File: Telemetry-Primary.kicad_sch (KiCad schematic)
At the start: 43 parts, among them J10 SDCard_LogicAnalyzer, J13 GPS_LogicAnalyzer, J5 SWD, J6 Breakouts, J7 CAN_LogicAnalyzer, J7 RTC_BATT, J8 CAN_LogicAnalyzer, SW1 Reset, U9 STM32F429ZITx, Y2 8M, Y3 32.768k

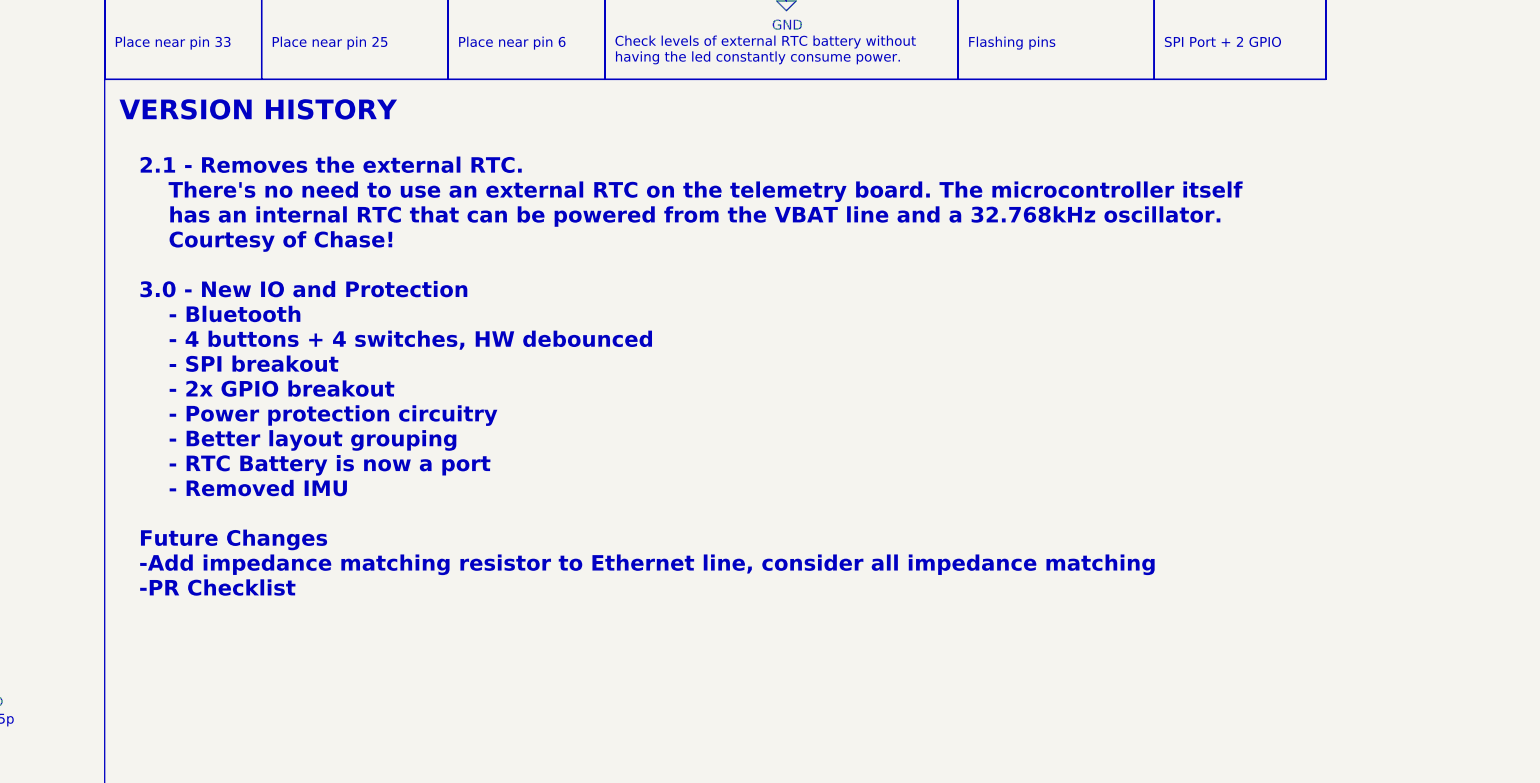
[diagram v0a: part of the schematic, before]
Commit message: silk screen cleanup + comments
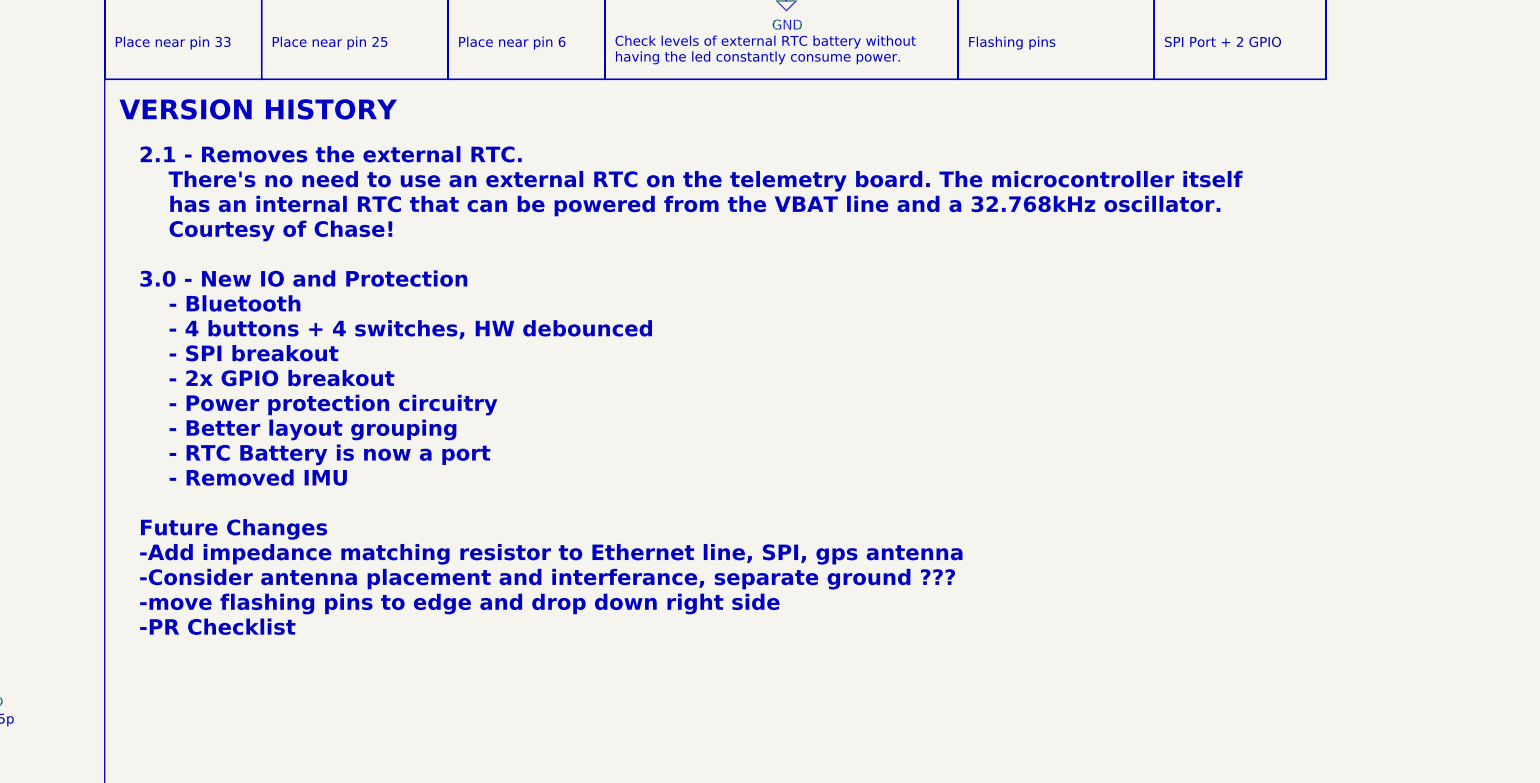
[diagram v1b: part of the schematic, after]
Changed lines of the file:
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@@
     (effects (font (size 1.27 1.27)) (justify left bottom))
   )
-  (text "2.1 - Removes the external RTC.\n	There's no need to use an external RTC on the telemetry board. The microcontroller itself\n	has an internal RTC that can be powered from the VBAT line and a 32.768kHz oscillator. \n	Courtesy of Chase!\n\n3.0 - New IO and Protection\n	- Bluetooth\n	- 4 buttons + 4 switches, HW debounced\n	- SPI breakout\n	- 2x GPIO breakout\n	- Power protection circuitry\n	- Better layout grouping\n	- RTC Battery is now a port\n	- Removed IMU\n\nFuture Changes\n-Add impedance matching resistor to Ethernet line, consider all impedance matching\n-PR Checklist"
-    (at 254 158.115 0)
+  (text "2.1 - Removes the external RTC.\n	There's no need to use an external RTC on the telemetry board. The microcontroller itself\n	has an internal RTC that can be powered from the VBAT line and a 32.768kHz oscillator. \n	Courtesy of Chase!\n\n3.0 - New IO and Protection\n	- Bluetooth\n	- 4 buttons + 4 switches, HW debounced\n	- SPI breakout\n	- 2x GPIO breakout\n	- Power protection circuitry\n	- Better layout grouping\n	- RTC Battery is now a port\n	- Removed IMU\n\nFuture Changes\n-Add impedance matching resistor to Ethernet line, SPI, gps antenna\n-Consider antenna placement and interferance, separate ground ???\n-move flashing pins to edge and drop down right side\n-PR Checklist"
+    (at 254 163.195 0)
     (effects (font (size 2 2) (thickness 0.4) bold) (justify left bottom))
   )
